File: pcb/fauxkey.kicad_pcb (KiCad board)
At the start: 2 copper layers, 58.5 x 26.3 mm, 0 parts

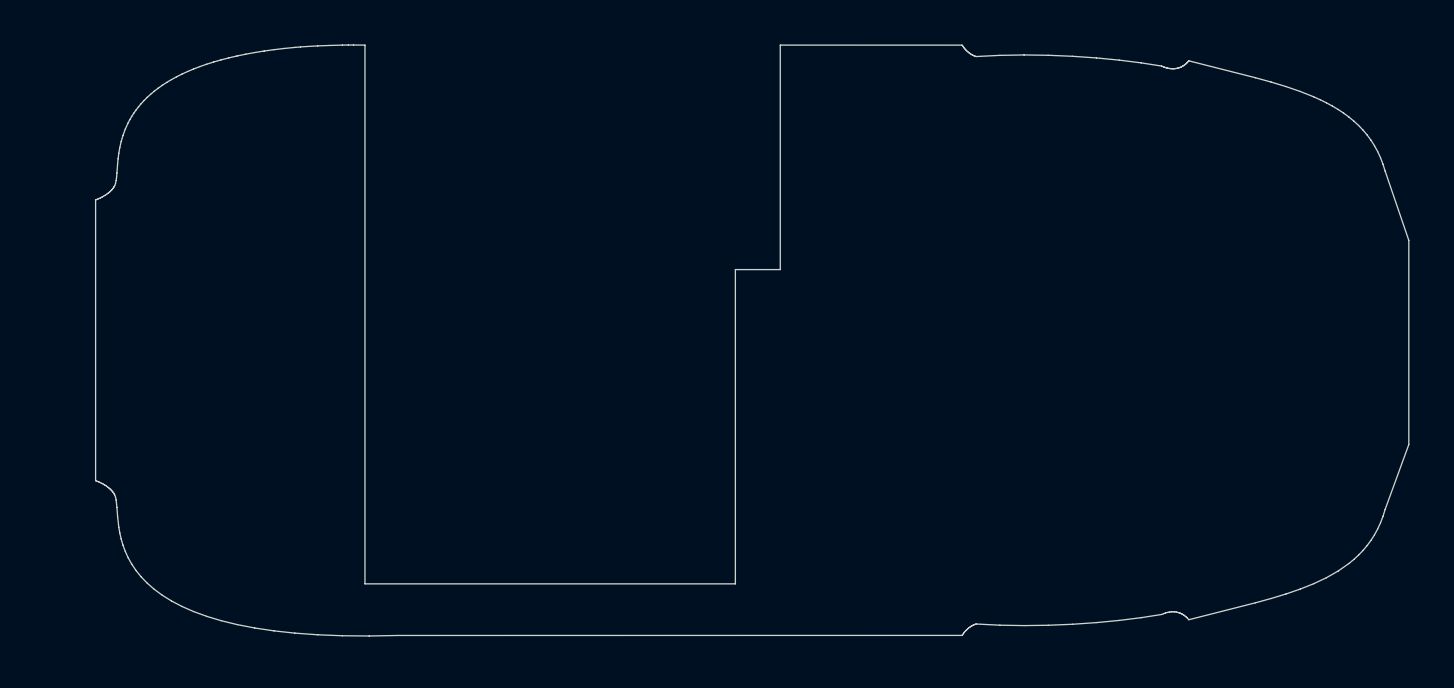
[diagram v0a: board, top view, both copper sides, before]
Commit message: Design PCB v0.1
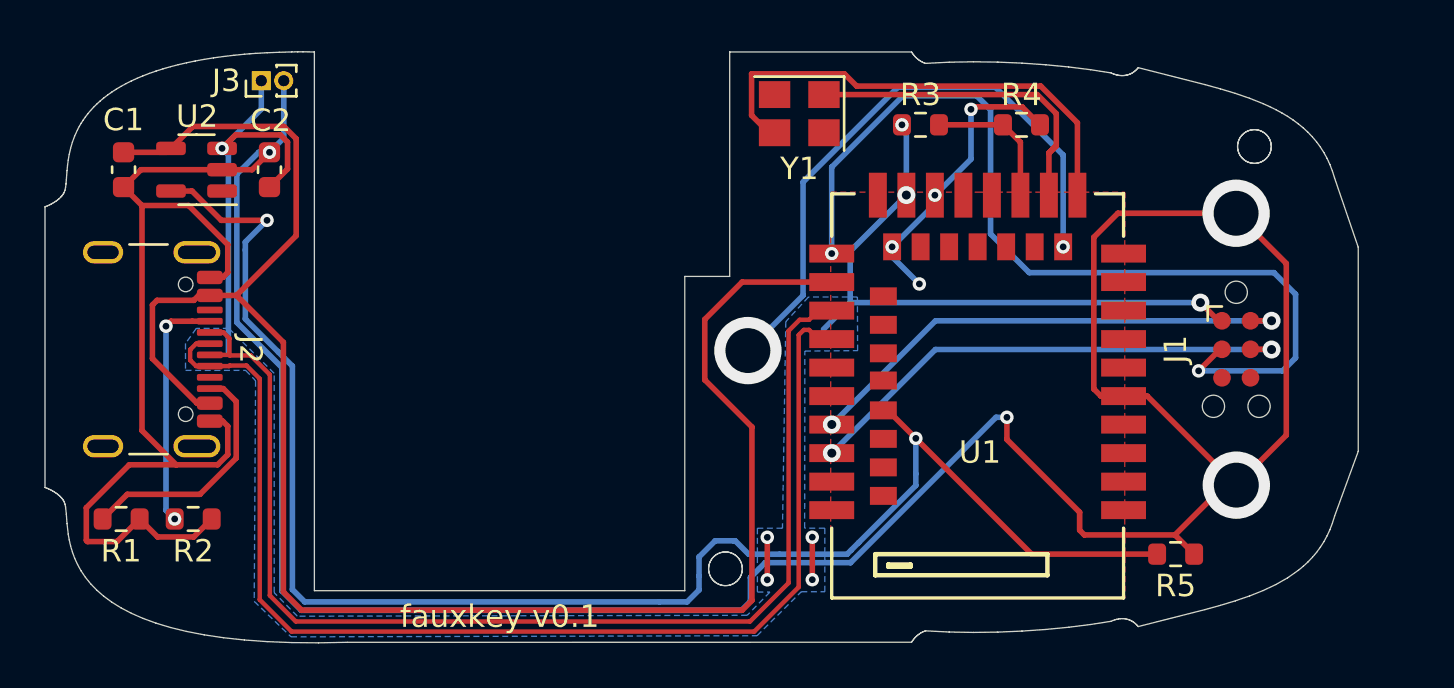
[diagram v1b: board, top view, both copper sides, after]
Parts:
- added C1: 10nF, Capacitor_SMD:C_0603_1608Metric, F.Cu at (120.0, 87.0)
- added C2: 10nF, Capacitor_SMD:C_0603_1608Metric, F.Cu at (126.5, 87.0)
- added J1: Conn_ARM_SWD_TagConnect_TC2030-NL, Connector:Tag-Connect_TC2030-IDC-NL_2x03_P1.27mm_Vertical, F.Cu at (169.6, 95.0)
- added J2: USB_C_Receptacle_USB2.0, Connector_USB:USB_C_Receptacle_GCT_USB4105-xx-A_16P_TopMnt_Horizontal, F.Cu at (120.2, 95.0)
- added J3: Conn_01x02, Connector_PinHeader_1.00mm:PinHeader_1x02_P1.00mm_Vertical, F.Cu at (126.1, 83.0)
- added R1: 5.1k, Resistor_SMD:R_0603_1608Metric, F.Cu at (119.9, 102.6)
- added R2: 5.1k, Resistor_SMD:R_0603_1608Metric, F.Cu at (123.1, 102.6)
- added R3: 800k, Resistor_SMD:R_0603_1608Metric, F.Cu at (155.5, 85.0)
- added R4: 2M, Resistor_SMD:R_0603_1608Metric, F.Cu at (160.0, 85.0)
- added R5: 2k, Resistor_SMD:R_0603_1608Metric, F.Cu at (166.9, 104.1)
- added U1: E73-2G4M08S1C, E73-2G4M08S1C:E73-2G4M08S1C, F.Cu at (158.0, 95.2)
- added U2: LTC4054ES5-4.2, Package_TO_SOT_SMD:TSOT-23-5, F.Cu at (123.2, 87.0)
- added Y1: 32.768 kHz, Crystal:Crystal_SMD_3225-4Pin_3.2x2.5mm, F.Cu at (150.1, 84.5)
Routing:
- net GND: track 0.00 -> 172.0 mm, vias 0 -> 8
- net /Power/USB_VBUS: track 0.00 -> 81.4 mm
- net /Power/PROG: track 0.00 -> 71.0 mm, vias 0 -> 2
- net /Power/USB_D+: track 0.00 -> 53.1 mm
- net /Power/USB_D-: track 0.00 -> 52.4 mm
- net /Power/VCC: track 0.00 -> 50.1 mm, vias 0 -> 8
- net Net-(J1-~{RESET}): track 0.00 -> 41.6 mm, vias 0 -> 2
- net unconnected-(U1-P0.26-Pad12): track 0.00 -> 27.2 mm, vias 0 -> 2
- net Net-(J1-SWCLK): track 0.00 -> 22.4 mm, vias 0 -> 2
- net Net-(J1-SWDIO): track 0.00 -> 22.4 mm, vias 0 -> 2
- net Net-(U1-P0.00/XL1): track 0.00 -> 21.8 mm
- net Net-(U1-P0.01/XL2): track 0.00 -> 14.9 mm
- net Net-(J2-CC2): track 0.00 -> 11.0 mm
- net Net-(J2-CC1): track 0.00 -> 10.8 mm, vias 0 -> 2
- net /Power/VCC_DIV: track 0.00 -> 6.31 mm
- added copper zone on B.Cu, net /Power/VCC
- added copper zone on F.Cu, net GND
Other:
- outline, holes or cut-outs redrawn
- board text added: "JLCJLCJLCJLC"
- board text added: "fauxkey v0.1"
